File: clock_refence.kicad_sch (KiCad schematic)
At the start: 140 parts, among them J201 REFIN, J202 REFIN_DIRECT_P, J203 REFIN_DIRECT_N, J204 REFOUT_AUX_P, J205 REFOUT_AUX_N, J206 RFShield_TwoPieces, J207 REFOUT, J208 VTUNE, J209 DNP, T201 TC2-1T+, T202 TC2-1T+, U201 Si53301, U202 XC6204B33, U203 TSV914, U204 74LVC1G66, X201 XTCLH40M000CHJA0P0

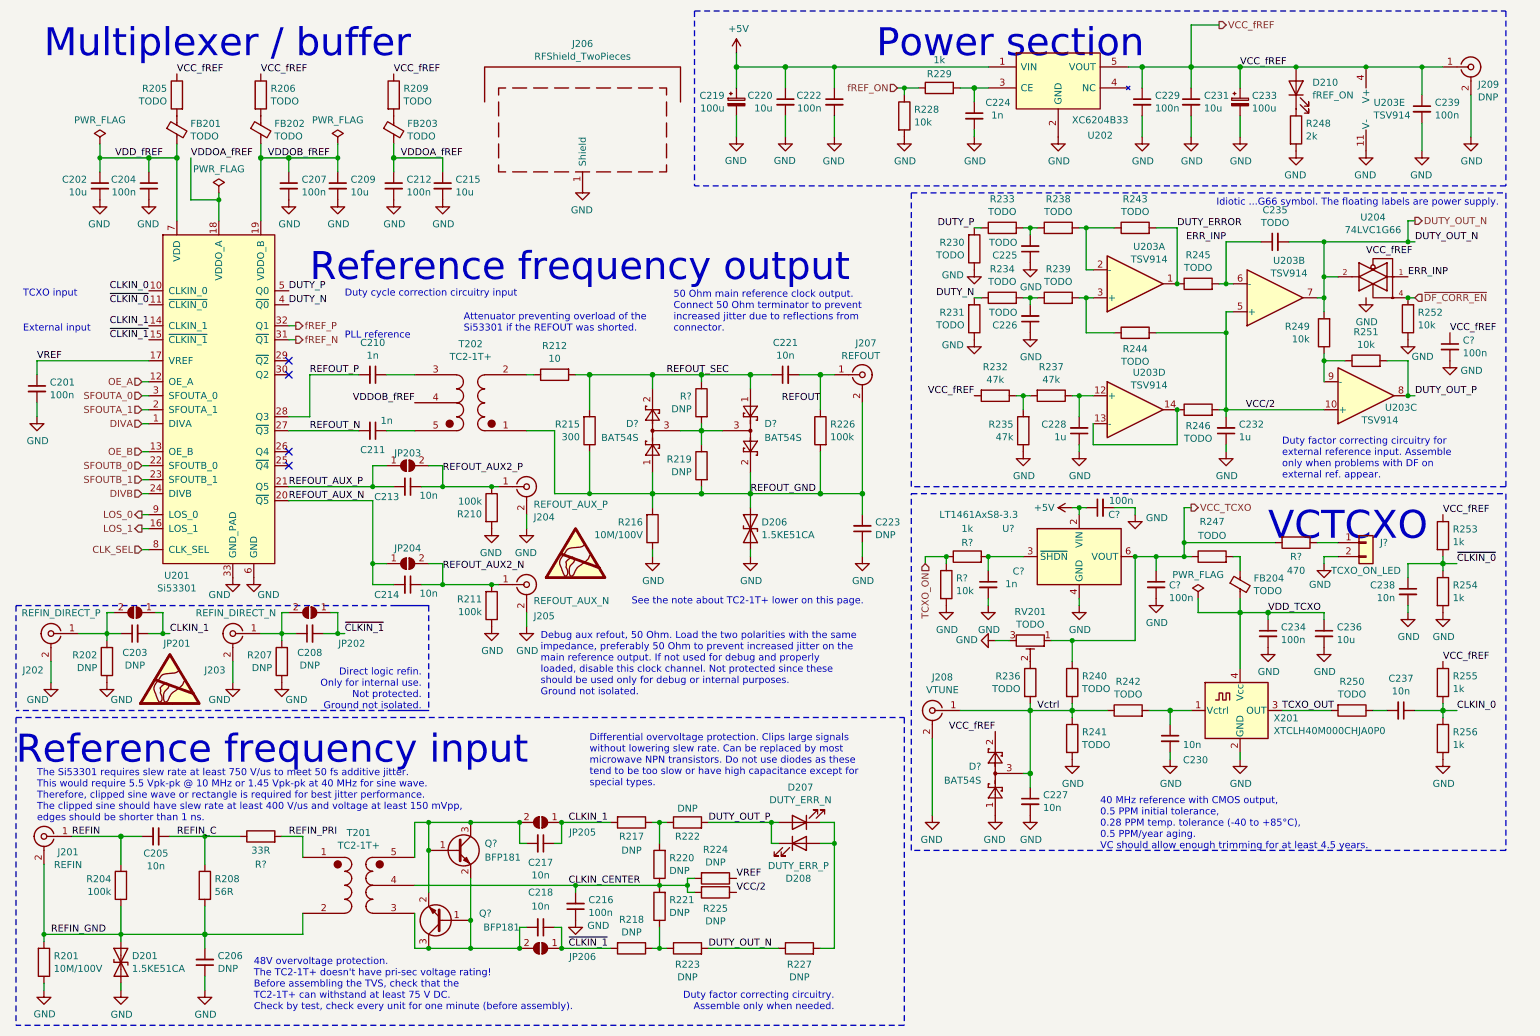
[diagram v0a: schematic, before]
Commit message: Updated schematics
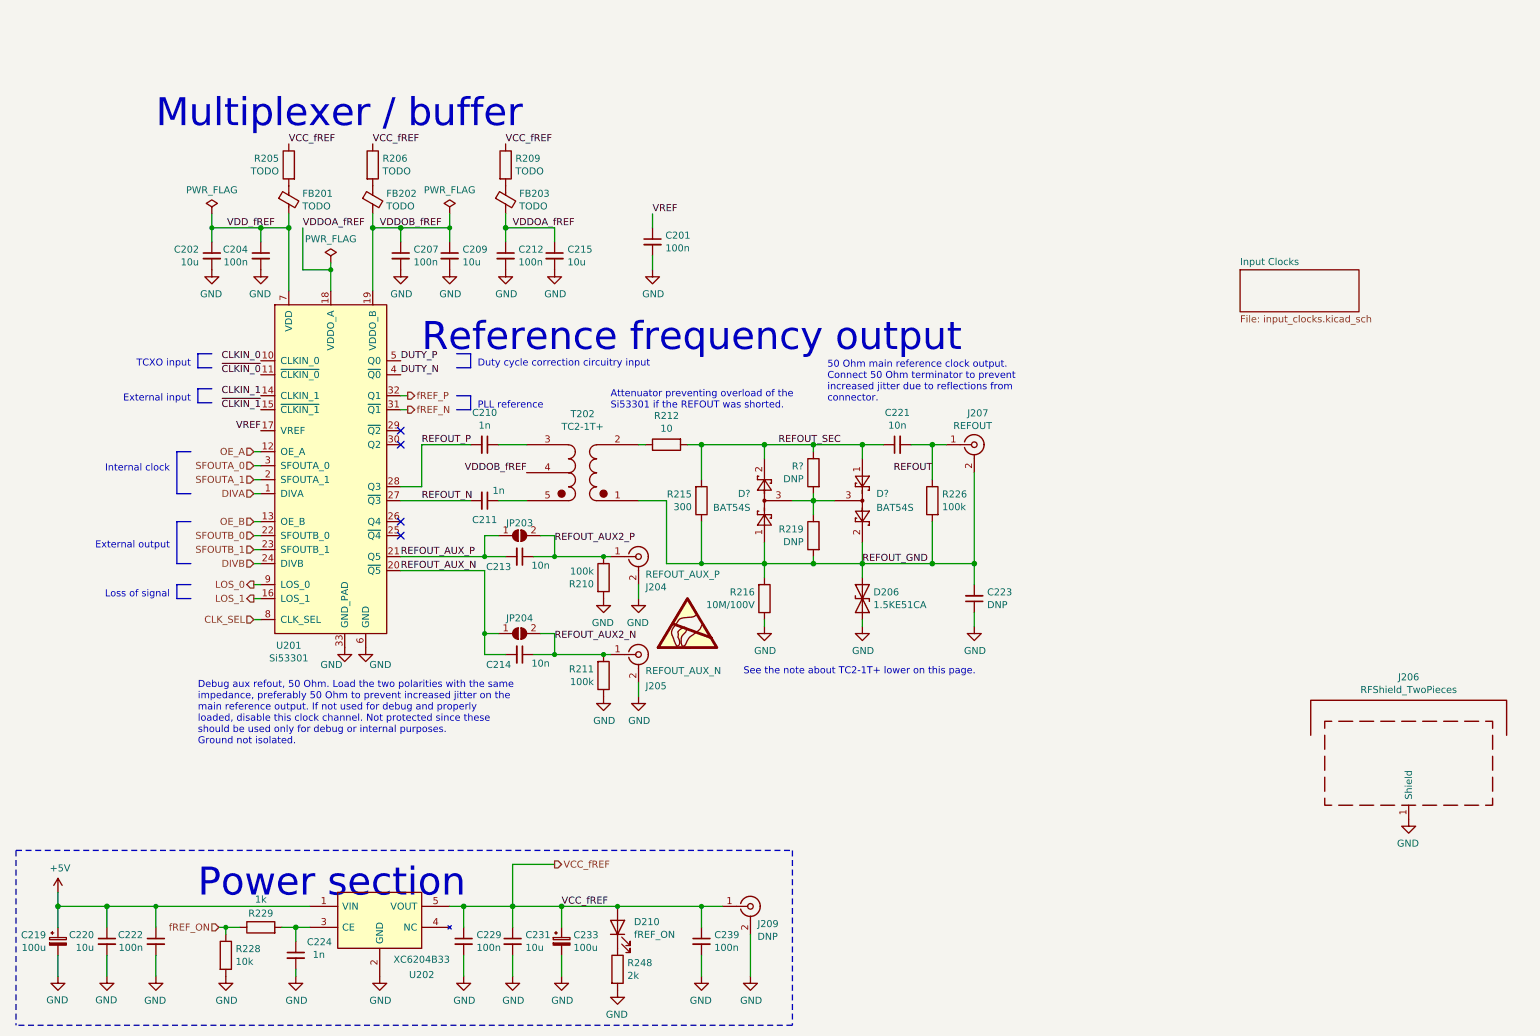
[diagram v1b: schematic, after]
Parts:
- removed C203, C206, C208: DNP, Capacitor_SMD:C_0603_1608Metric_Pad1.08x0.95mm_HandSolder, symbol Device:C_Small
- removed C205, C217, C218, C227, C230, C237, C238: 10n, Capacitor_SMD:C_0603_1608Metric_Pad1.08x0.95mm_HandSolder, symbol Device:C_Small
- removed C216, C234, C? (x3): 100n, Capacitor_SMD:C_0603_1608Metric_Pad1.08x0.95mm_HandSolder, symbol Device:C_Small
- removed C225, C226, C235: TODO, Capacitor_SMD:C_0603_1608Metric_Pad1.08x0.95mm_HandSolder, symbol Device:C_Small
- removed C228, C232: 1u, Capacitor_SMD:C_0603_1608Metric_Pad1.08x0.95mm_HandSolder, symbol Device:C_Small
- removed C236: 10u, Capacitor_SMD:C_0805_2012Metric_Pad1.18x1.45mm_HandSolder, symbol Device:C_Small
- removed C?: 1n, Capacitor_SMD:C_0603_1608Metric_Pad1.08x0.95mm_HandSolder, symbol Device:C_Small
- removed D201: 1.5KE51CA, Diode_THT:D_DO-201AE_P15.24mm_Horizontal, symbol Diode:1.5KExxCA
- removed D207: DUTY_ERR_N, LED_SMD:LED_0603_1608Metric_Pad1.05x0.95mm_HandSolder, symbol Device:LED
- removed D208: DUTY_ERR_P, LED_SMD:LED_0603_1608Metric_Pad1.05x0.95mm_HandSolder, symbol Device:LED
- removed D?: BAT54S, Package_TO_SOT_SMD:SOT-23, symbol Diode:BAT54S
- removed FB204: TODO, Inductor_SMD:L_0603_1608Metric_Pad1.05x0.95mm_HandSolder, symbol Device:FerriteBead_Small
- removed J201: REFIN, petr_kicad:SMA_rosenberger_hybrid, symbol Connector:Conn_Coaxial
- removed J202: REFIN_DIRECT_P, petr_kicad:SMA_rosenberger_hybrid, symbol Connector:Conn_Coaxial
- removed J203: REFIN_DIRECT_N, petr_kicad:SMA_rosenberger_hybrid, symbol Connector:Conn_Coaxial
- removed J208: VTUNE, petr_kicad:SMA_rosenberger_hybrid, symbol Connector:Conn_Coaxial
- removed J?: TCXO_ON_LED, symbol Connector_Generic:Conn_01x02
- removed JP201, JP202, JP205, JP206: SolderJumper_2_Open, Jumper:SolderJumper-2_P1.3mm_Open_RoundedPad1.0x1.5mm, symbol Jumper:SolderJumper_2_Open
- removed Q? (x2): BFP181, Package_TO_SOT_SMD:SOT-23_Handsoldering, symbol petr:BFP181
- removed R201: 10M/100V, Resistor_SMD:R_1206_3216Metric_Pad1.30x1.75mm_HandSolder, symbol Device:R
- removed R202, R207, R217, R218, R220, R221, R222, R223, R224, R225, R227: DNP, Resistor_SMD:R_0603_1608Metric_Pad0.98x0.95mm_HandSolder, symbol Device:R
- removed R204: 100k, Resistor_SMD:R_0603_1608Metric_Pad0.98x0.95mm_HandSolder, symbol Device:R
- removed R208: 56R, Resistor_SMD:R_0603_1608Metric_Pad0.98x0.95mm_HandSolder, symbol Device:R
- removed R230, R231, R233, R234, R236, R238, R239, R240, R241, R242, R243, R244, R245, R246, R247, R250: TODO, Resistor_SMD:R_0603_1608Metric_Pad0.98x0.95mm_HandSolder, symbol Device:R
- removed R232, R235, R237: 47k, Resistor_SMD:R_0603_1608Metric_Pad0.98x0.95mm_HandSolder, symbol Device:R
- removed R249, R251, R252, R?: 10k, Resistor_SMD:R_0603_1608Metric_Pad0.98x0.95mm_HandSolder, symbol Device:R
- removed R253, R254, R255, R256, R?: 1k, Resistor_SMD:R_0603_1608Metric_Pad0.98x0.95mm_HandSolder, symbol Device:R
- removed R?: 33R, Resistor_SMD:R_0603_1608Metric_Pad0.98x0.95mm_HandSolder, symbol Device:R
- removed R?: 470, Resistor_SMD:R_0603_1608Metric_Pad0.98x0.95mm_HandSolder, symbol Device:R
- removed RV201: TODO, Potentiometer_THT:Potentiometer_Bourns_3296Y_Vertical, symbol Device:R_Potentiometer_Trim
- removed T201: TC2-1T+, Transformer_SMD:Transformer_MACOM_SM-22, symbol petr_lib_nightly:TC2-1T+
- removed U203: TSV914, Package_SO:SOIC-14_3.9x8.7mm_P1.27mm, symbol Amplifier_Operational:TSV914
- removed U204: 74LVC1G66, Package_TO_SOT_SMD:SOT-353_SC-70-5_Handsoldering, symbol 74xGxx:74LVC1G66
- removed U?: LT1461AxS8-3.3, Package_SO:SOIC-8_3.9x4.9mm_P1.27mm, symbol Reference_Voltage:LT1461AxS8-3.3
- removed X201: XTCLH40M000CHJA0P0, Oscillator:Oscillator_SMD_Fordahl_DFAS15-4Pin_5.0x3.2mm_HandSoldering, symbol petr_lib_nightly:XTCLH40M000CHJA0P0
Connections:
- net VCC renamed VCC_fREF
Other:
- added sheet Input Clocks (input_clocks.kicad_sch)
- note added: "External output"
- note added: "Internal clock"
- note added: "Loss of signal"
- note removed: "40 MHz reference with CMOS output, 0.5 PPM initial tolerance, 0.28 PPM temp. tolerance (-40 to +85°C), 0.5 PPM/year aging. VC should allow enough trimming for at least 4.5 years."
- note removed: "48V overvoltage protection. The TC2-1T+ doesn't have pri-sec voltage rating! Before assembling the TVS, check that the TC2-1T+ can withstand at least 75 V DC. Check by test, check every unit for one minute (before assembly)."
- note removed: "Differential overvoltage protection. Clips large signals without lowering slew rate. Can be replaced by most microwave NPN transistors. Do not use diodes as these tend to be too slow or have high capacitance except for special types."
- note removed: "Direct logic refin. Only for internal use. Not protected. Ground not isolated."
- note removed: "Duty factor correcting circuitry for external reference input. Assemble only when problems with DF on external ref. appear."
- note removed: "Duty factor correcting circuitry. Assemble only when needed."
- note removed: "Idiotic ...G66 symbol. The floating labels are power supply."
- note removed: "Reference frequency input"
- note removed: "The Si53301 requires slew rate at least 750 V/us to meet 50 fs additive jitter. This would require 5.5 Vpk-pk @ 10 MHz or 1.45 Vpk-pk at 40 MHz for sine wave. Therefore, clipped sine wave or rectangle is required for best jitter performance. The clipped sine should have slew rate at least 400 V/us and voltage at least 150 mVpp, edges should be shorter than 1 ns."
- note removed: "VCTCXO"
- moved on the sheet: C201, C202, C204, C207, C209, C210, C211, C212, C213, C214, C215, C219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
